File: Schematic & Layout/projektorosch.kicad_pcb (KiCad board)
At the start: 2 copper layers, 39 parts, among them J1 Power barrel plug, J2 RJ12, U1 ATmega328-P, U2 MAX232, Y1 Crystal

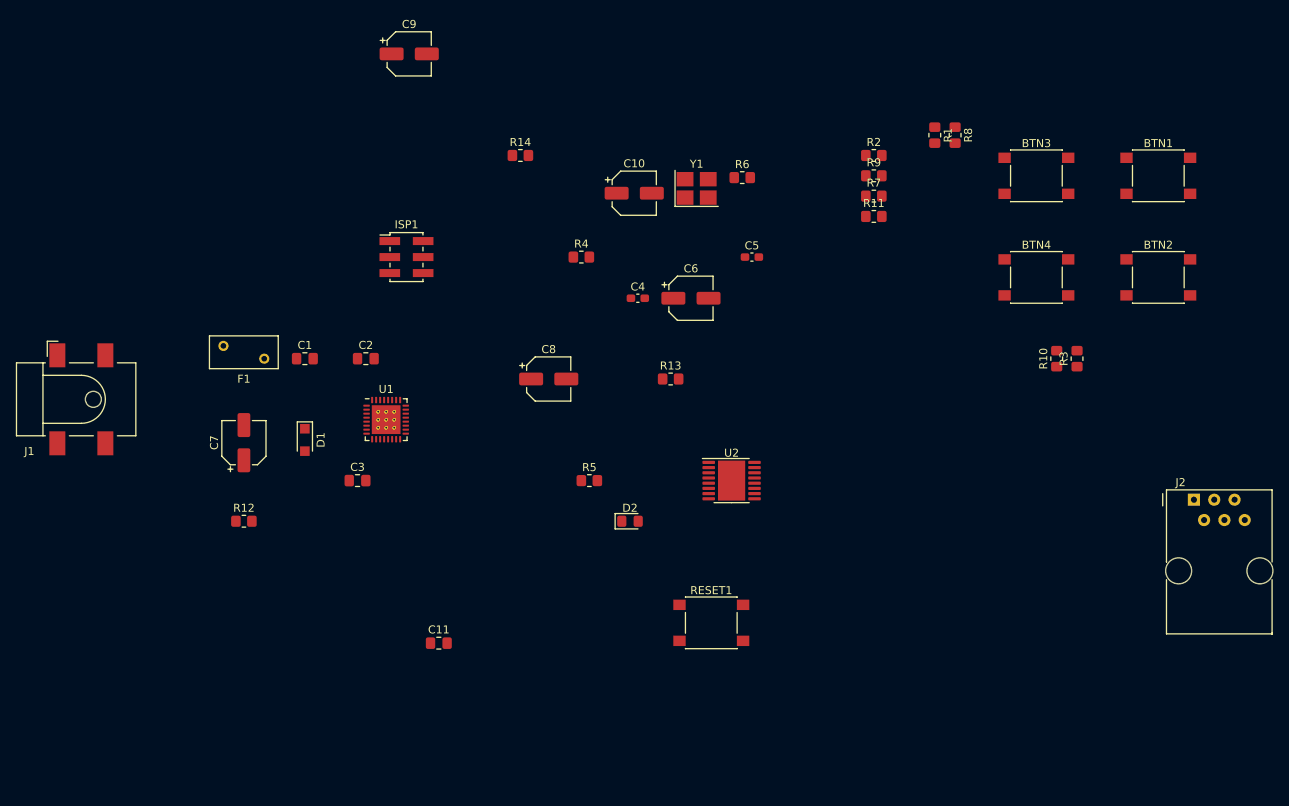
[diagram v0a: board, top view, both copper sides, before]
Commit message: design pcb - first try
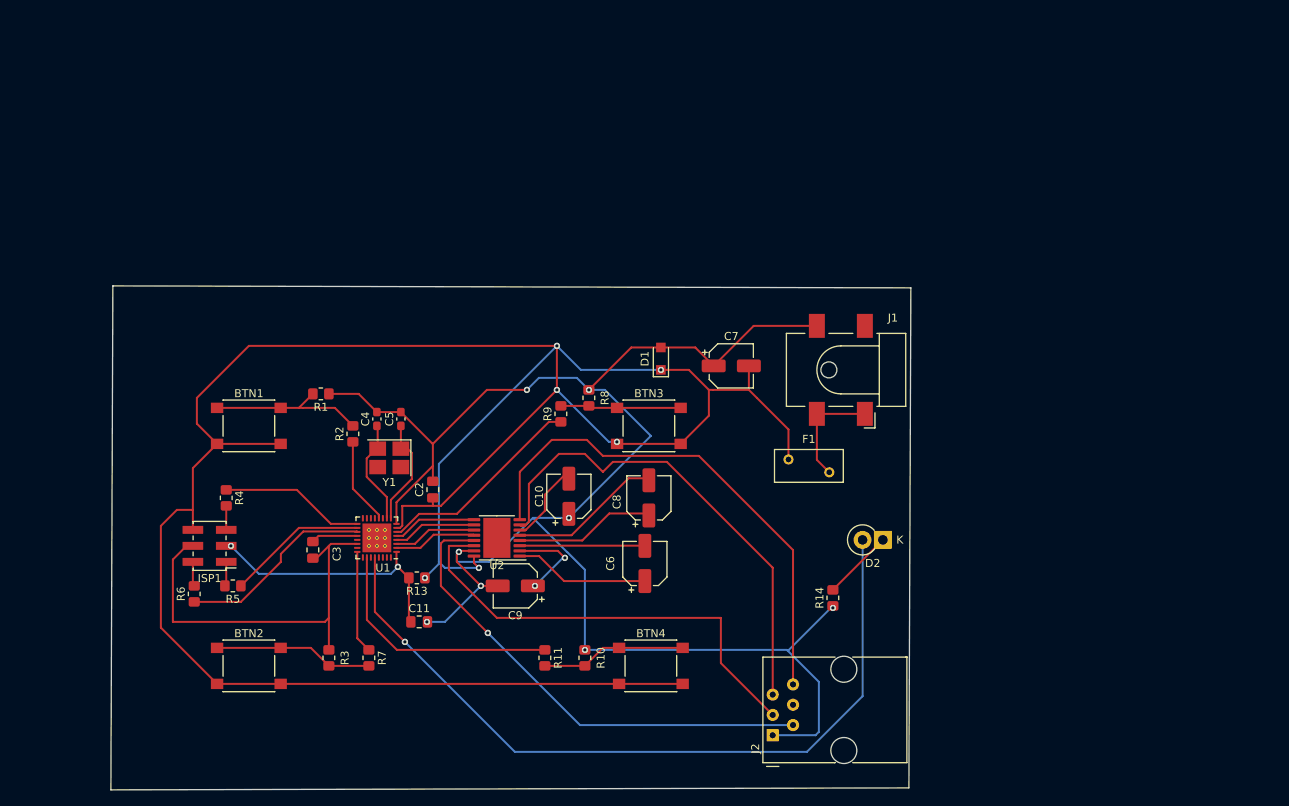
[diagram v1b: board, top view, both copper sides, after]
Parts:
- removed C1: 100nF, Capacitor_SMD:C_0805_2012Metric_Pad1.18x1.45mm_HandSolder
- removed R12: R, Resistor_SMD:R_0805_2012Metric_Pad1.20x1.40mm_HandSolder
- removed RESET1: SW_SPST, Button_Switch_SMD:SW_Push_1P1T_NO_6x6mm_H9.5mm
- D2: footprint Diode_SMD:D_0805_2012Metric_Pad1.15x1.40mm_HandSolder -> Diode_THT:D_DO-15_P2.54mm_Vertical_KathodeUp
- moved BTN2 123.6 mm to (120.0, 140.0)
- moved BTN1 117.9 mm to (120.0, 110.0)
- moved R3 100.7 mm to (130.0, 139.0), turned to -90 degrees
- moved J1 95.0 mm to (194.0, 103.0), turned to 180 degrees
- moved R6 86.0 mm to (113.2, 131.0), turned to 90 degrees
- moved R7 85.5 mm to (135.0, 139.0), turned to -90 degrees
- moved R1 83.3 mm to (129.0, 106.0), turned to 180 degrees
- moved R2 73.8 mm to (133.0, 111.0), turned to 90 degrees
- moved R10 69.8 mm to (162.0, 139.0), turned to -90 degrees
- moved R11 68.8 mm to (157.0, 139.0), turned to -90 degrees
- moved BTN4 68.4 mm to (170.2, 140.0)
- moved C9 67.8 mm to (153.3, 130.0), turned to 180 degrees
- moved R14 67.7 mm to (193.0, 131.5), turned to 90 degrees
- moved F1 66.7 mm to (187.4, 114.2), turned to 0 degrees
- moved C7 61.7 mm to (180.3, 102.5), turned to 0 degrees
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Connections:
- J2 pad 1: /RX -> GND
- J2 pad 3: GND -> /RX
- J2 pad 5: /RTS -> /CTS
- J2 pad 6: /CTS -> /RTS
- U1 pad 12: unconnected-(U1-Pad12) -> BTN1
- U1 pad 2: /TX -> Net-(U1-Pad2)
- U1 pad 21: Net-(C1-Pad1) -> unconnected-(U1-Pad21)
- U1 pad 23: BTN1 -> unconnected-(U1-Pad23)
- U1 pad 25: BTN3 -> unconnected-(U1-Pad25)
- U1 pad 28: unconnected-(U1-Pad28) -> Net-(D2-Pad2)
- U1 pad 6: Net-(D2-Pad2) -> BTN3
- U2 pad 12: /TX -> Net-(U1-Pad2)
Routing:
- net VCC: track 0.00 -> 310.1 mm, vias 0 -> 6
- net GND: track 0.00 -> 267.3 mm, vias 0 -> 8
- net Net-(D2-Pad2): track 0.00 -> 97.4 mm, vias 0 -> 1
- net /RTS: track 0.00 -> 64.3 mm
- net /CTS: track 0.00 -> 61.7 mm
- net /TX: track 0.00 -> 61.0 mm, vias 0 -> 1
- net /RX: track 0.00 -> 57.4 mm
- net !RESET: track 0.00 -> 32.5 mm, vias 0 -> 2
- net BTN4: track 0.00 -> 31.6 mm
- net BTN3: track 0.00 -> 26.2 mm
- net Net-(R6-Pad1): track 0.00 -> 24.6 mm
- net Net-(BTN1-Pad1): track 0.00 -> 20.4 mm
- net Net-(BTN2-Pad1): track 0.00 -> 19.9 mm
- net Net-(C8-Pad2): track 0.00 -> 19.1 mm
- net Net-(R4-Pad1): track 0.00 -> 18.1 mm
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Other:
- board outline added: 100 x 63 mm
